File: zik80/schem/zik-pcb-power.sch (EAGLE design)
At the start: 9 parts, among them IC1 TPS7133QP, IC2 7805TV

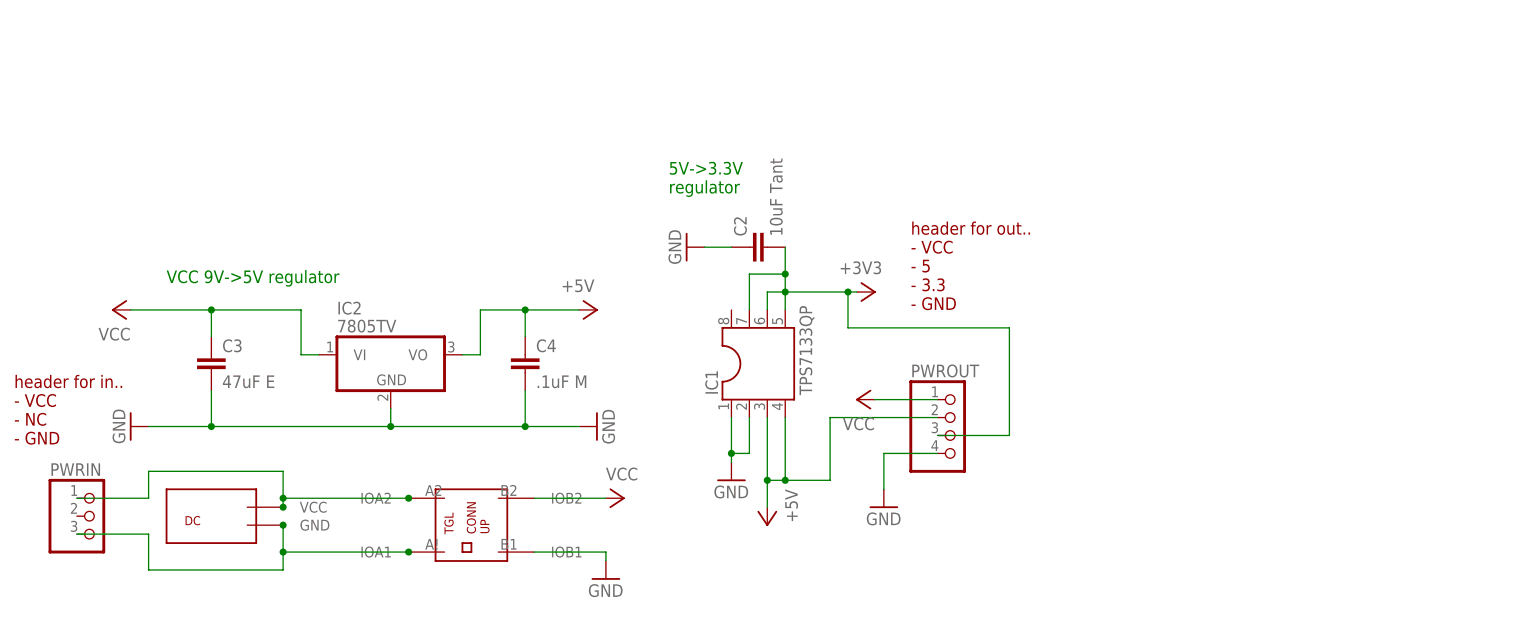
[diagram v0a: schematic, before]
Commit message: minor tweaks to gpu sche.. getting mentally ready for finishing it up, deciding what is pinheader versus actual footprints..
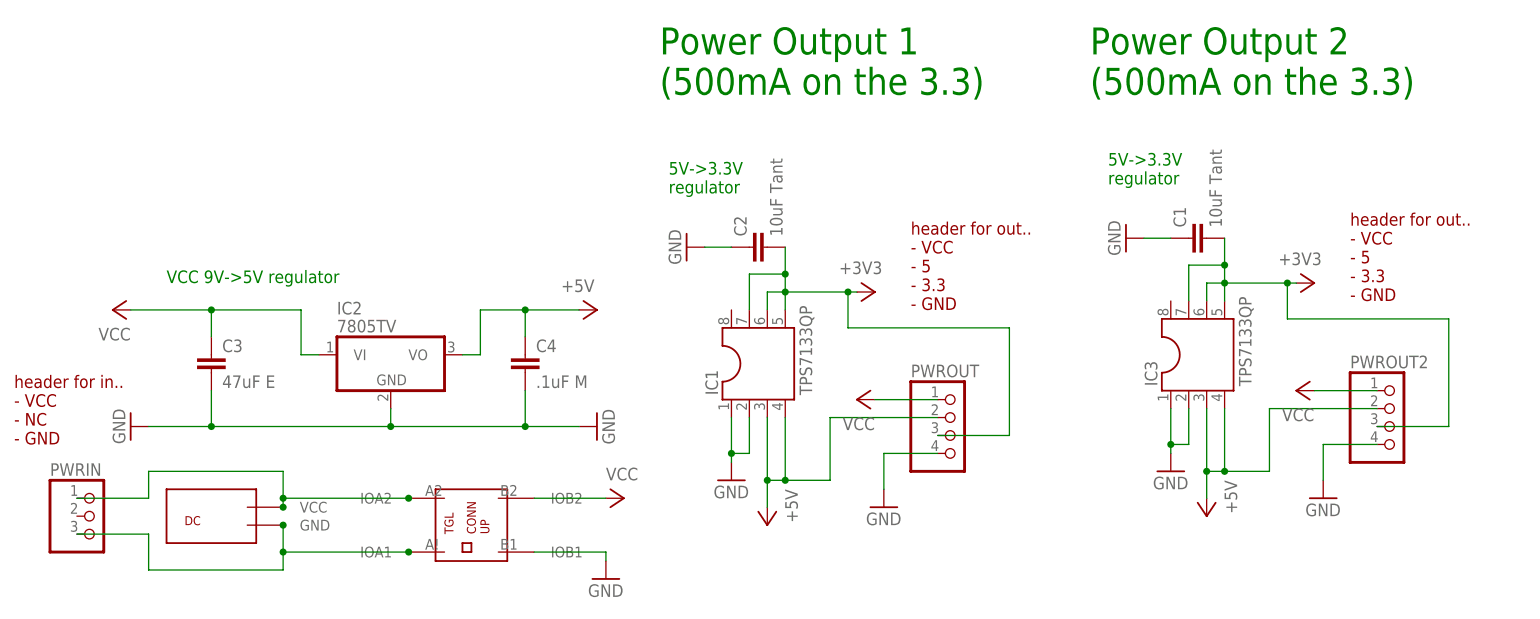
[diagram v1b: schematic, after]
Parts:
- added C1: 10uF Tant, rcl:C-EU025-025X050
- added IC3: TPS7133QP, ic-package:DIL8
- added PWROUT2: (no value), pinhead:PINHD-1X4
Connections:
- net +3V3: now also C1.2, IC3.5, IC3.6, IC3.7, PWROUT2.3
- net +5V: now also IC3.3, IC3.4, PWROUT2.2
- net GND: now also C1.1, IC3.1, IC3.2, PWROUT2.4
- net VCC: now also PWROUT2.1
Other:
- note added: "Power Output 1 (500mA on the 3.3)"
- note added: "Power Output 2 (500mA on the 3.3)"
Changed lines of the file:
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@@
 <part name="GND1" library="supply1" deviceset="GND" device=""/>
 <part name="P+1" library="supply1" deviceset="VCC" device=""/>
+<part name="IC3" library="ic-package" deviceset="DIL8" device="" value="TPS7133QP"/>
+<part name="GND7" library="supply1" deviceset="GND" device=""/>
+<part name="P+6" library="supply1" deviceset="+5V" device=""/>
+<part name="C1" library="rcl" deviceset="C-EU" device="025-025X050" value="10uF Tant"/>
+<part name="GND8" library="supply1" deviceset="GND" device=""/>
+<part name="+3V2" library="supply1" deviceset="+3V3" device=""/>
+<part name="PWROUT2" library="pinhead" deviceset="PINHD-1X4" device=""/>
+<part name="GND9" library="supply1" deviceset="GND" device=""/>
+<part name="P+7" library="supply1" deviceset="VCC" device=""/>
 </parts>
 <sheets>
@@
 - NC
 - GND</text>
+<text x="135.89" y="38.1" size="1.778" layer="91">5V-&gt;3.3V
+regulator</text>
+<text x="170.18" y="21.59" size="1.778" layer="94">header for out..
+- VCC
+- 5
+- 3.3
+- GND</text>
+<text x="72.39" y="50.8" size="3.81" layer="91">Power Output 1
+(500mA on the 3.3)</text>
+<text x="133.35" y="50.8" size="3.81" layer="91">Power Output 2
+(500mA on the 3.3)</text>
 </plain>
 <instances>
@@
 <instance part="GND1" gate="1" x="104.14" y="-7.62"/>
 <instance part="P+1" gate="VCC" x="100.33" y="7.62" rot="R90"/>
+<instance part="IC3" gate="G$1" x="147.32" y="13.97" rot="R90"/>
+<instance part="GND7" gate="1" x="144.78" y="-2.54"/>
+<instance part="P+6" gate="1" x="149.86" y="-8.89" rot="R180"/>
+<instance part="C1" gate="G$1" x="147.32" y="30.48" rot="R90"/>
+<instance part="GND8" gate="1" x="138.43" y="30.48" rot="R270"/>
+<instance part="+3V2" gate="G$1" x="165.1" y="24.13" rot="R270"/>
+<instance part="PWROUT2" gate="A" x="176.53" y="3.81"/>
+<instance part="GND9" gate="1" x="166.37" y="-6.35"/>
+<instance part="P+7" gate="VCC" x="162.56" y="8.89" rot="R90"/>
 </instances>
 <busses>
@@
 <junction x="53.34" y="20.32"/>
 <pinref part="P+4" gate="1" pin="+5V"/>
+</segment>
+<segment>
+<pinref part="IC3" gate="G$1" pin="3"/>
+<pinref part="P+6" gate="1" pin="+5V"/>
+<wire x1="149.86" y1="6.35" x2="149.86" y2="-2.54" width="0.1524" layer="91"/>
+<pinref part="IC3" gate="G$1" pin="4"/>
+<wire x1="149.86" y1="-2.54" x2="149.86" y2="-6.35" width="0.1524" layer="91"/>
+<wire x1="152.4" y1="6.35" x2="152.4" y2="-2.54" width="0.1524" layer="91"/>
+<wire x1="152.4" y1="-2.54" x2="149.86" y2="-2.54" width="0.1524" layer="91"/>
+<junction x="149.86" y="-2.54"/>
+<wire x1="152.4" y1="-2.54" x2="158.75" y2="-2.54" width="0.1524" layer="91"/>
+<wire x1="158.75" y1="-2.54" x2="158.75" y2="6.35" width="0.1524" layer="91"/>
+<junction x="152.4" y="-2.54"/>
+<pinref part="PWROUT2" gate="A" pin="2"/>
+<wire x1="158.75" y1="6.35" x2="173.99" y2="6.35" width="0.1524" layer="91"/>
 </segment>
 </net>
@@
 <wire x1="104.14" y1="0" x2="104.14" y2="-5.08" width="0.1524" layer="91"/>
 <pinref part="GND1" gate="1" pin="GND"/>
+</segment>
+<segment>
+<pinref part="IC3" gate="G$1" pin="1"/>
+<pinref part="GND7" gate="1" pin="GND"/>
+<wire x1="144.78" y1="6.35" x2="144.78" y2="1.27" width="0.1524" layer="91"/>
+<pinref part="IC3" gate="G$1" pin="2"/>
+<wire x1="144.78" y1="1.27" x2="144.78" y2="0" width="0.1524" layer="91"/>
+<wire x1="147.32" y1="6.35" x2="147.32" y2="1.27" width="0.1524" layer="91"/>
+<wire x1="147.32" y1="1.27" x2="144.78" y2="1.27" width="0.1524" layer="91"/>
+<junction x="144.78" y="1.27"/>
+</segment>
+<segment>
+<pinref part="C1" gate="G$1" pin="1"/>
+<wire x1="144.78" y1="30.48" x2="140.97" y2="30.48" width="0.1524" layer="91"/>
+<pinref part="GND8" gate="1" pin="GND"/>
+</segment>
+<segment>
+<pinref part="PWROUT2" gate="A" pin="4"/>
+<wire x1="173.99" y1="1.27" x2="166.37" y2="1.27" width="0.1524" layer="91"/>
+<wire x1="166.37" y1="1.27" x2="166.37" y2="-3.81" width="0.1524" layer="91"/>
+<pinref part="GND9" gate="1" pin="GND"/>
 </segment>
 </net>
@@
 <wire x1="121.92" y1="2.54" x2="111.76" y2="2.54" width="0.1524" layer="91"/>
 </segment>
+<segment>
+<pinref part="IC3" gate="G$1" pin="5"/>
+<pinref part="C1" gate="G$1" pin="2"/>
+<wire x1="152.4" y1="21.59" x2="152.4" y2="24.13" width="0.1524" layer="91"/>
+<pinref part="IC3" gate="G$1" pin="7"/>
+<wire x1="152.4" y1="24.13" x2="152.4" y2="26.67" width="0.1524" layer="91"/>
+<wire x1="152.4" y1="26.67" x2="152.4" y2="30.48" width="0.1524" layer="91"/>
+<wire x1="152.4" y1="26.67" x2="147.32" y2="26.67" width="0.1524" layer="91"/>
+<wire x1="147.32" y1="26.67" x2="147.32" y2="21.59" width="0.1524" layer="91"/>
+<junction x="152.4" y="26.67"/>
+<pinref part="IC3" gate="G$1" pin="6"/>
+<wire x1="152.4" y1="24.13" x2="149.86" y2="24.13" width="0.1524" layer="91"/>
+<wire x1="149.86" y1="24.13" x2="149.86" y2="21.59" width="0.1524" layer="91"/>
+<junction x="152.4" y="24.13"/>
+<wire x1="152.4" y1="24.13" x2="161.29" y2="24.13" width="0.1524" layer="91"/>
+<pinref part="+3V2" gate="G$1" pin="+3V3"/>
+<wire x1="161.29" y1="24.13" x2="162.56" y2="24.13" width="0.1524" layer="91"/>
+<wire x1="161.29" y1="24.13" x2="161.29" y2="19.05" width="0.1524" layer="91"/>
+<wire x1="161.29" y1="19.05" x2="184.15" y2="19.05" width="0.1524" layer="91"/>
+<wire x1="184.15" y1="19.05" x2="184.15" y2="3.81" width="0.1524" layer="91"/>
+<junction x="161.29" y="24.13"/>
+<pinref part="PWROUT2" gate="A" pin="3"/>
+<wire x1="184.15" y1="3.81" x2="173.99" y2="3.81" width="0.1524" layer="91"/>
+</segment>
 </net>
 <net name="VCC" class="0">
@@
 <pinref part="P+1" gate="VCC" pin="VCC"/>
 </segment>
-</net>
+<segment>
+<pinref part="PWROUT2" gate="A" pin="1"/>
+<wire x1="173.99" y1="8.89" x2="165.1" y2="8.89" width="0.1524" layer="91"/>
+<pinref part="P+7" gate="VCC" pin="VCC"/>
+</segment>
+</net>
